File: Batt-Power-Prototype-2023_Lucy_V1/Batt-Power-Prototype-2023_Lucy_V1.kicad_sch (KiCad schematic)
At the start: 49 parts, among them IC1 ESDALC6V1W5, J1 GPIO, J14 DE9_Receptacle_MountingHoles, J4 USB_B_Micro, J8 OLED, SW1 SW_SPDT, SW2 RESET, U1 STM32L432KCUx, U10 8MHz, U10 MCP2542FD-E/SN, U7 FT234XD-R

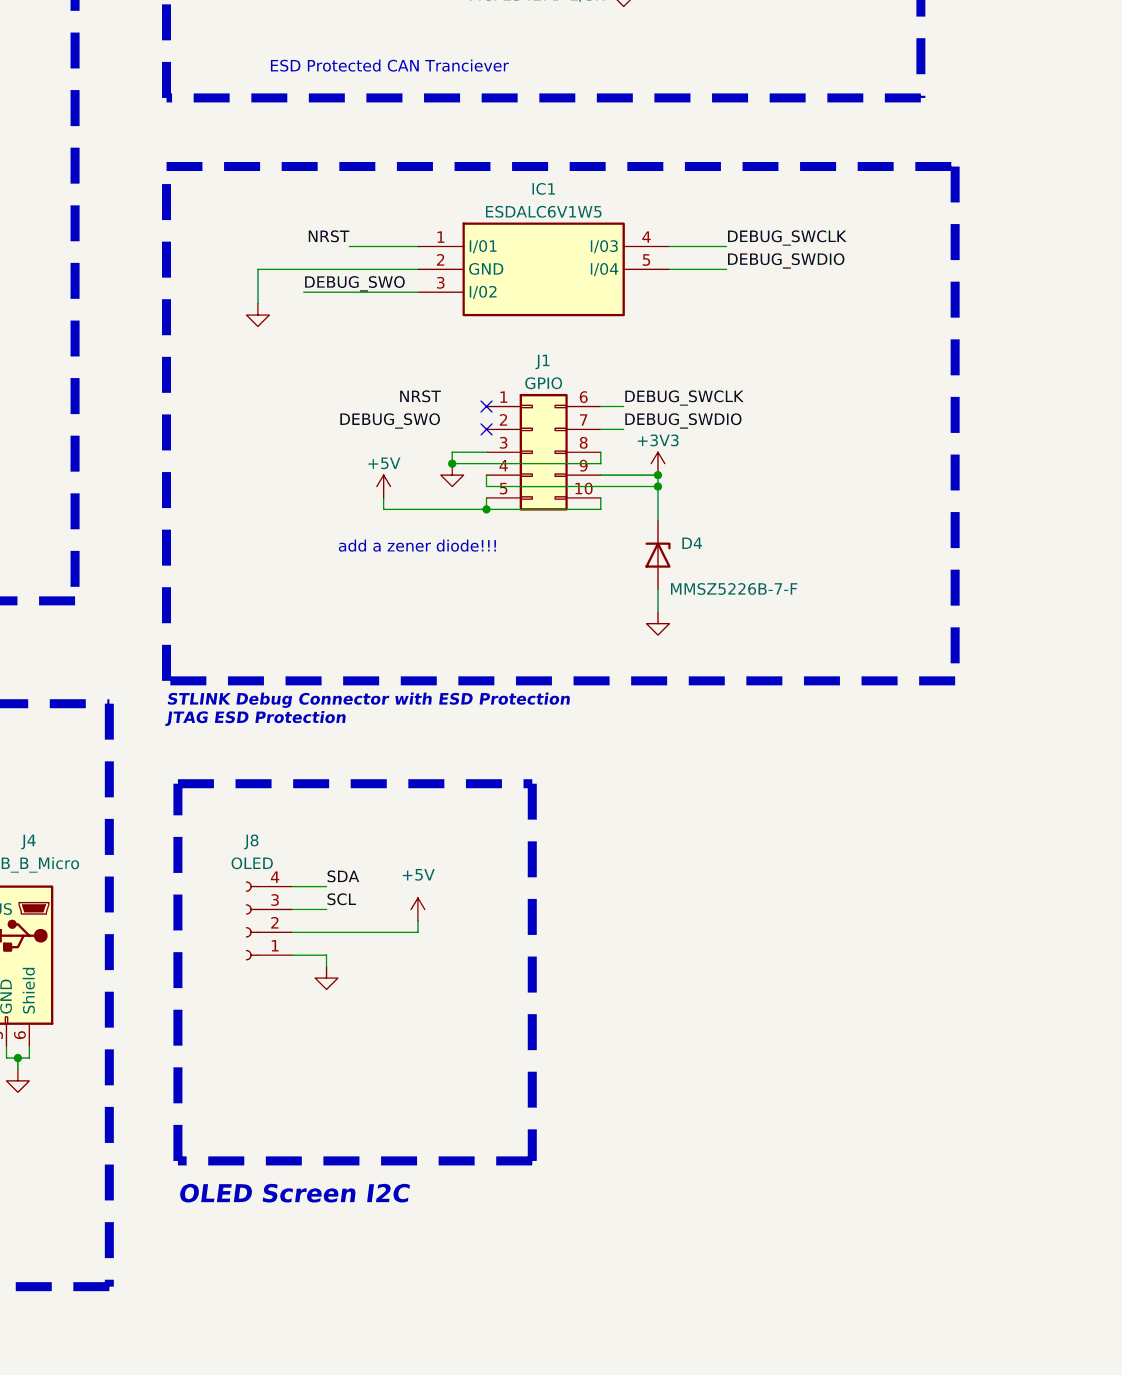
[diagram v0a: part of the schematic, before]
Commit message: schematic done??
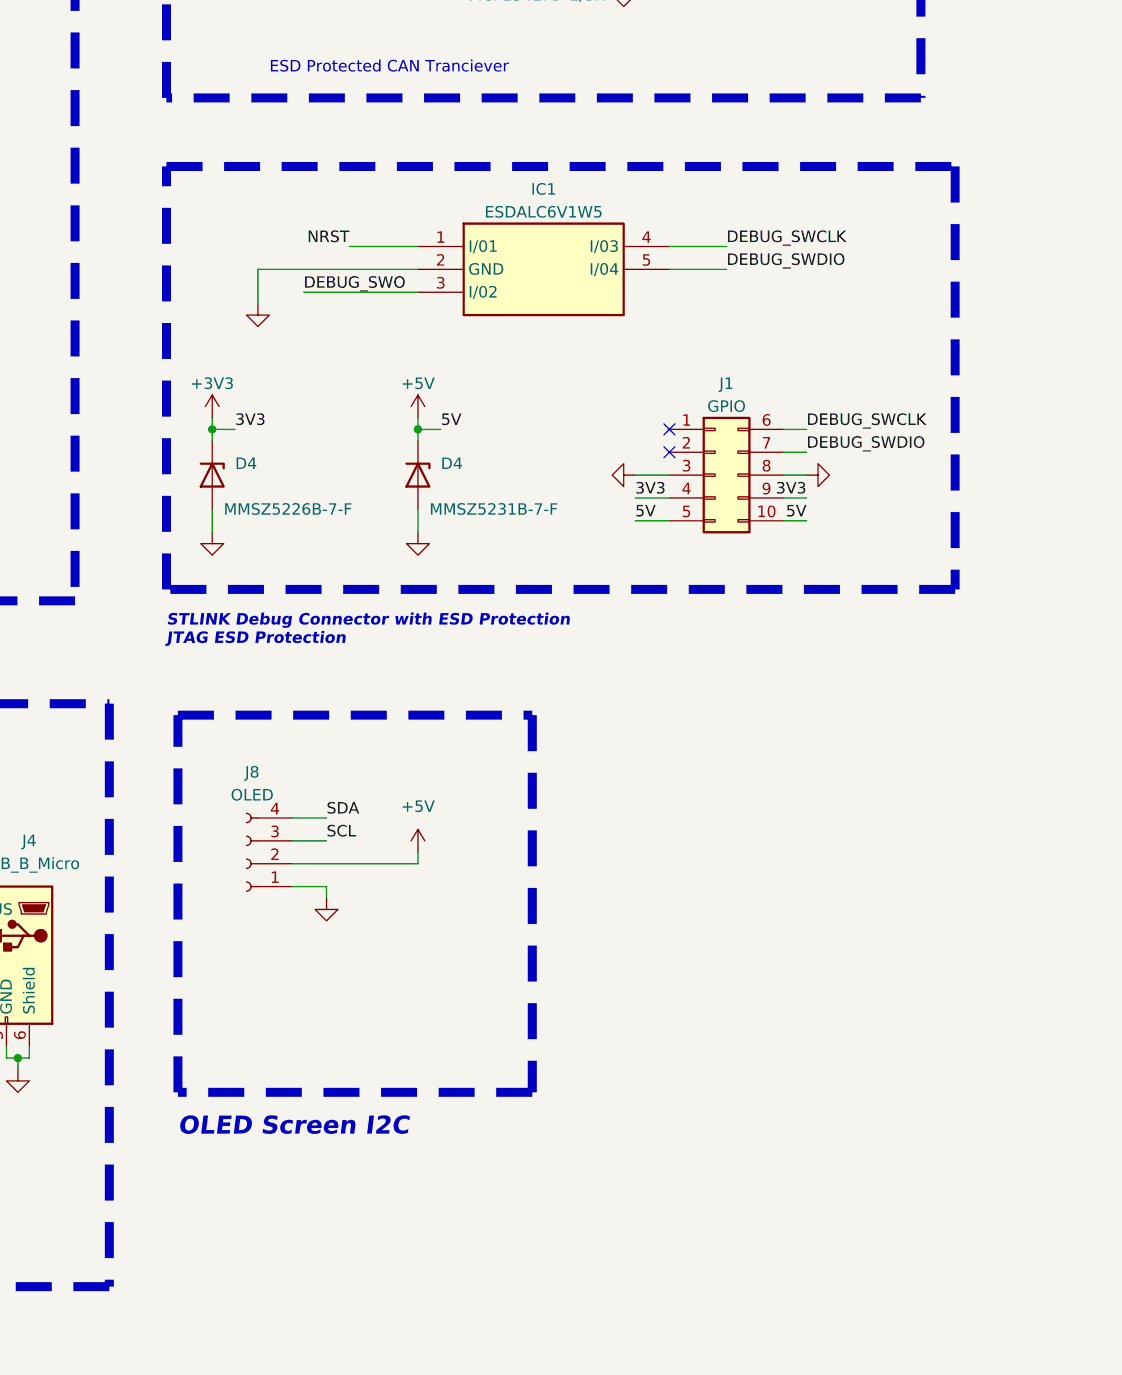
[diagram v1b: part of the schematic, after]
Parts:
- added D4: MMSZ5231B-7-F, Diode_SMD:D_SOD-123, symbol Device:D_Zener
- IC1: footprint SYM&FOOT:SOT65P210X110-5N -> BP_FTP:SOT65P210X110-5N
- J14: footprint (none) -> Connector_Dsub:DSUB-9_Female_Horizontal_P2.77x2.84mm_EdgePinOffset7.70mm_Housed_MountingHolesOffset9.12mm
- J8: footprint SYM&FOOT:Display_128x64_096_I2C -> BP_FTP:Display_128x64_096_I2C
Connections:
- net +5V: now also D4.1 (K)
- net GND: now also D4.2 (A)
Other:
- note removed: "add a zener diode!!!"
- moved on the sheet: D4, J1, J8
